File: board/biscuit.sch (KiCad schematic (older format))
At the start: 59 parts

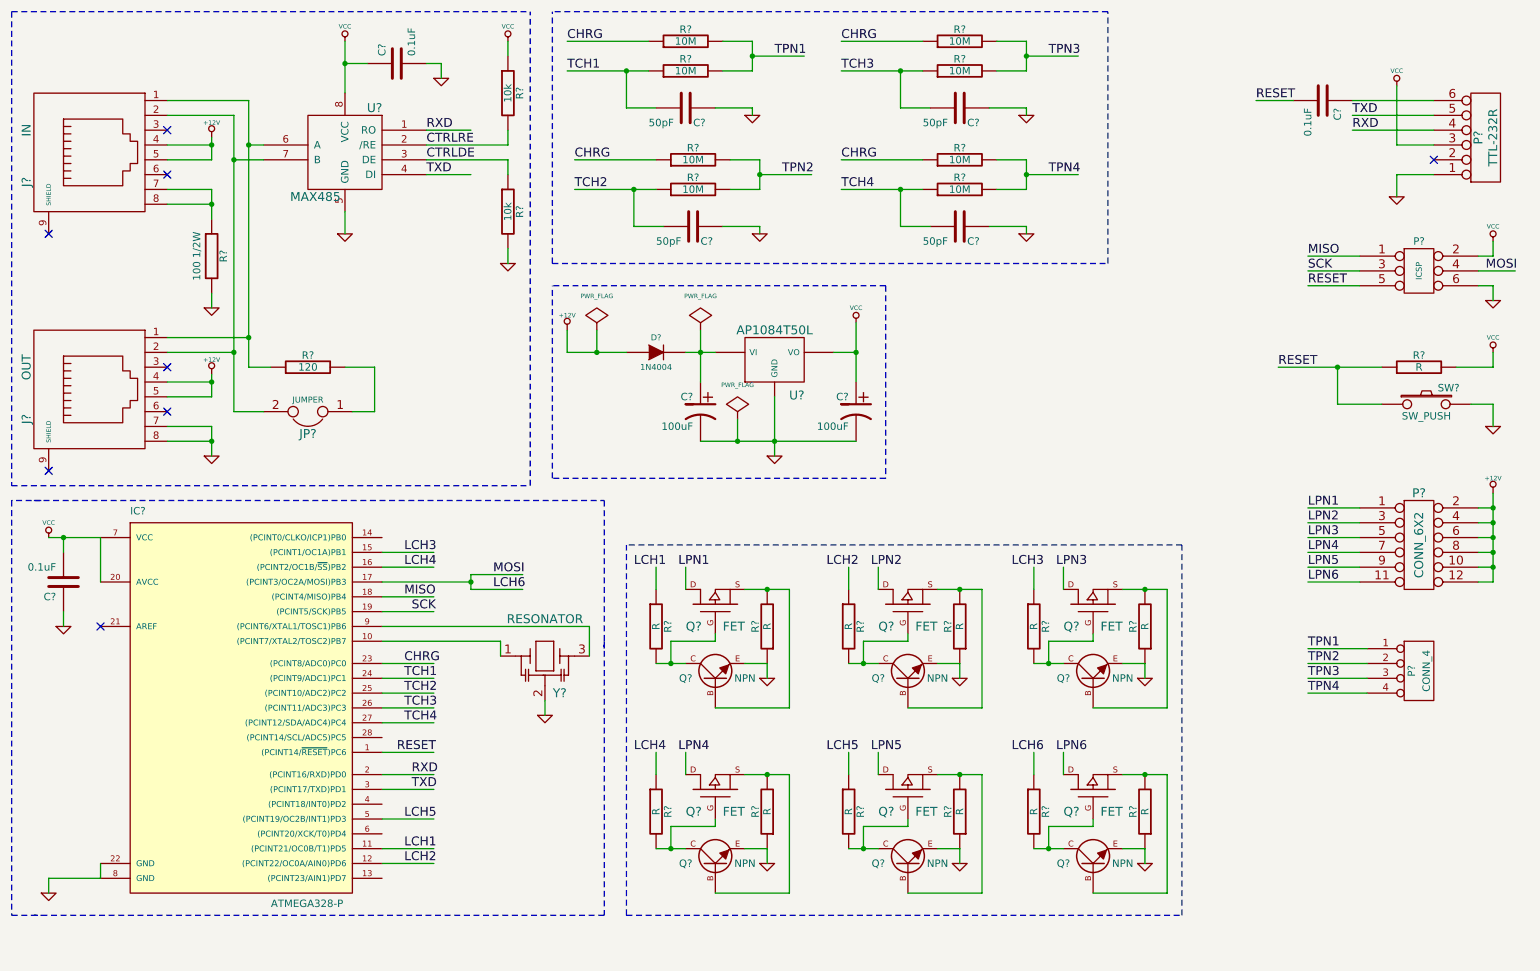
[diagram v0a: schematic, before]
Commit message: v1 of board
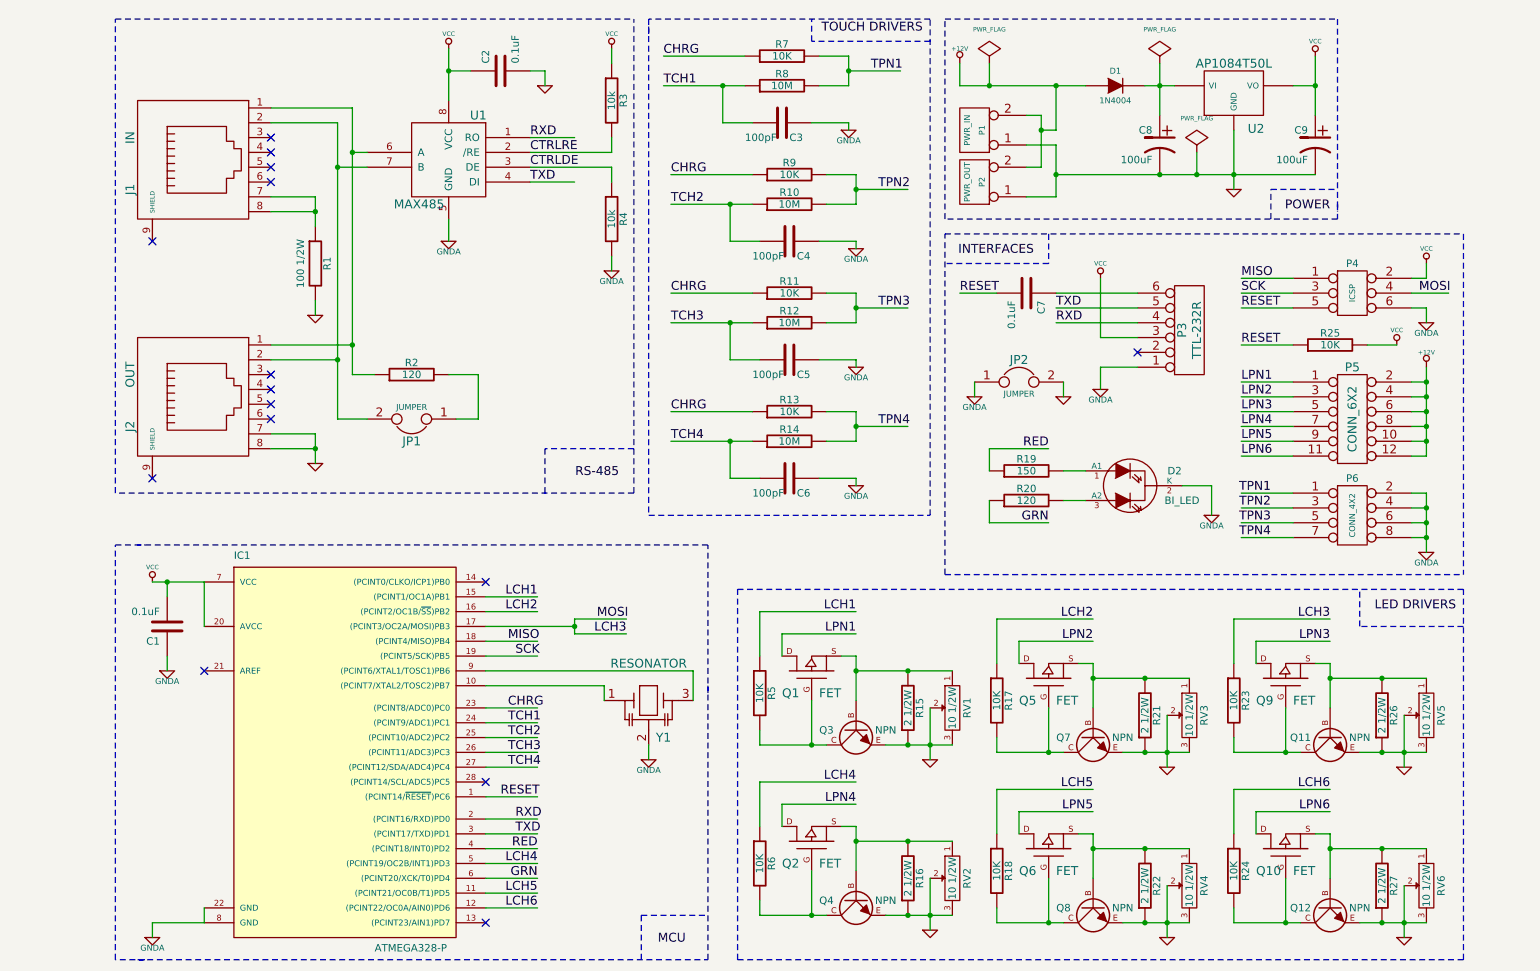
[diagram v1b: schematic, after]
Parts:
- removed P?: CONN_4, symbol CONN_4
- removed Q? (x6): FET, symbol MOSFET_P
- removed Q? (x6): NPN, TO92-EBC, symbol BC237
- removed R? (x12): R, symbol R
- removed SW?: SW_PUSH, symbol SW_PUSH
- added D2: BI_LED, symbol BI_LED
- added JP2: JUMPER, symbol JUMPER
- added P1: PWR_IN, symbol CONN_2
- added P2: PWR_OUT, symbol CONN_2
- added P6: CONN_4X2, symbol CONN_4X2
- added Q1, Q10, Q2, Q5, Q6, Q9: FET, symbol MOSFET_P
- added Q11, Q12, Q3, Q4, Q7, Q8: NPN, TO92-EBC, symbol BC237
- added R15, R16, R21, R22, R26, R27: 2 1/2W, symbol R
- added R17, R18, R23, R24, R5, R6: 10K, symbol R
- added R19: 150, symbol R
- added R20: 120, symbol R
- added RV1, RV2, RV3, RV4, RV5, RV6: 10 1/2W, symbol POT
- C3, C4, C5, C6: renamed from C?; value 50pF -> 100pF
- R11, R13, R7, R9: renamed from R?; value 10M -> 10K
- R25: renamed from R?; value R -> 10K
- gave numbers to parts that had none: 24
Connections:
- net labels added: GNDA, GRN, INTERFACES, LED DRIVERS, MCU, POWER, RED, RS-485, TOUCH DRIVERS
- wire segments 226 -> 246
- no-connect marks 8 -> 15
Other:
- moved on the sheet: C1, C2, C3, C4, C5, C6, C7, C8, C9, D1, IC1, J1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
